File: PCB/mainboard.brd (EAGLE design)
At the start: 80.3 x 68.6 mm, 22 parts, among them IC1 74LS42N, IC2 74HC147N

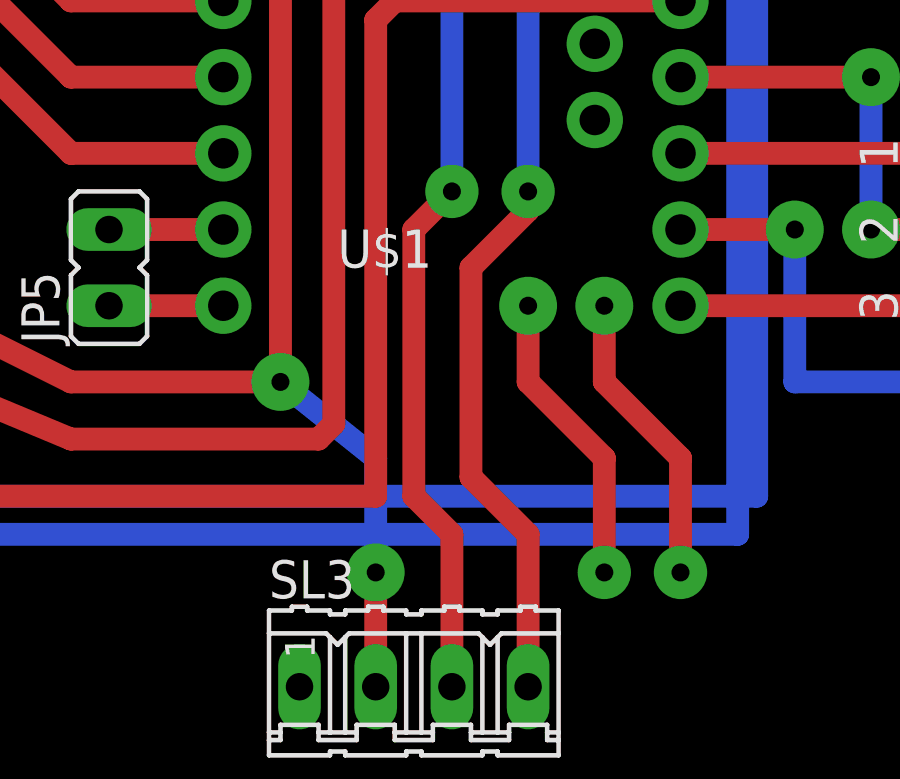
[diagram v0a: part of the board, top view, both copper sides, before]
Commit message: Modified sketch
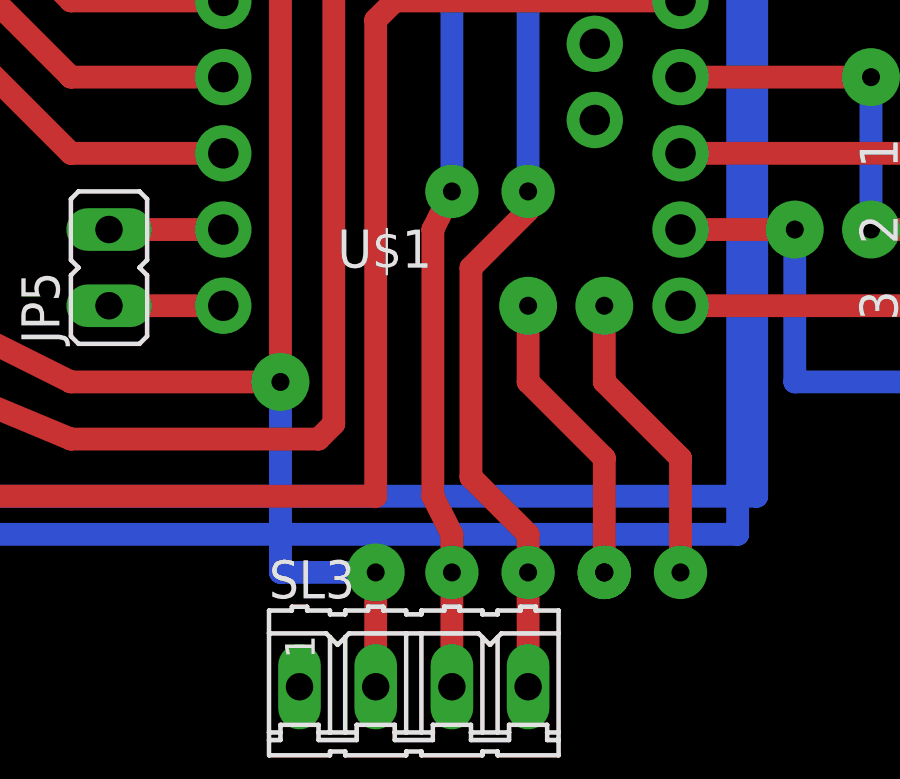
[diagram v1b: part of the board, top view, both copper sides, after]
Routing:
- net VCC: track 242.9 -> 244.6 mm
- net N$29: track 35.2 -> 34.4 mm
- net N$28: vias 4 -> 7
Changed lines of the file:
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@@
 <wire x1="63.5" y1="22.86" x2="63.5" y2="26.67" width="0.762" layer="1"/>
 <via x="63.5" y="26.67" extent="1-16" drill="0.6" diameter="1.9304"/>
-<wire x1="63.5" y1="26.67" x2="63.5" y2="30.48" width="0.762" layer="16"/>
-<wire x1="63.5" y1="30.48" x2="60.325" y2="33.02" width="0.762" layer="16"/>
+<wire x1="63.5" y1="26.67" x2="60.325" y2="26.67" width="0.762" layer="16"/>
+<wire x1="60.325" y1="26.67" x2="60.325" y2="33.02" width="0.762" layer="16"/>
 <via x="60.325" y="33.02" extent="1-16" drill="0.6" diameter="1.9304"/>
 </signal>
@@
 <wire x1="69.85" y1="54.61" x2="70.64375" y2="54.61" width="0.762" layer="1"/>
 <wire x1="70.64375" y1="54.61" x2="70.8025" y2="54.76875" width="0.762" layer="1"/>
-<wire x1="71.12" y1="26.67" x2="68.58" y2="22.86" width="0" layer="19" extent="1-1"/>
-<wire x1="73.66" y1="26.67" x2="71.12" y2="26.67" width="0" layer="19" extent="1-1"/>
 <wire x1="68.58" y1="52.07" x2="68.58" y2="39.37" width="0.762" layer="16"/>
 <wire x1="68.58" y1="39.37" x2="68.58" y2="38.735" width="0.762" layer="1"/>
@@
 <wire x1="66.675" y1="29.845" x2="68.58" y2="27.94" width="0.762" layer="1"/>
 <wire x1="68.58" y1="27.94" x2="68.58" y2="22.86" width="0.762" layer="1"/>
+<via x="68.58" y="26.67" extent="1-16" drill="0.6" diameter="1.778"/>
+<via x="71.12" y="26.67" extent="1-16" drill="0.6" diameter="1.778"/>
+<via x="66.04" y="26.67" extent="1-16" drill="0.6" diameter="1.778"/>
+<wire x1="71.12" y1="26.67" x2="73.66" y2="26.67" width="0" layer="19" extent="1-1"/>
+<wire x1="68.58" y1="26.67" x2="71.12" y2="26.67" width="0" layer="19" extent="1-1"/>
+<wire x1="68.58" y1="27.94" x2="68.58" y2="26.67" width="0" layer="19" extent="1-1"/>
+<wire x1="66.04" y1="26.67" x2="68.58" y2="26.67" width="0" layer="19" extent="1-1"/>
 </signal>
 <signal name="N$29">
@@
 <wire x1="70.8025" y1="50.165" x2="66.04" y2="50.165" width="0.762" layer="1"/>
 <wire x1="66.04" y1="50.165" x2="66.04" y2="39.37" width="0.762" layer="16"/>
-<wire x1="66.04" y1="39.37" x2="64.77" y2="38.1" width="0.762" layer="1"/>
-<wire x1="64.77" y1="38.1" x2="64.77" y2="29.21" width="0.762" layer="1"/>
-<wire x1="64.77" y1="29.21" x2="66.04" y2="27.94" width="0.762" layer="1"/>
+<wire x1="66.04" y1="39.37" x2="65.405" y2="38.1" width="0.762" layer="1"/>
+<wire x1="65.405" y1="38.1" x2="65.405" y2="29.21" width="0.762" layer="1"/>
+<wire x1="65.405" y1="29.21" x2="66.04" y2="27.94" width="0.762" layer="1"/>
 <wire x1="66.04" y1="27.94" x2="66.04" y2="22.86" width="0.762" layer="1"/>
 </signal>
